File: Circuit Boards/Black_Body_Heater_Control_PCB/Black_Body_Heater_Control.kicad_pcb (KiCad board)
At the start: 2 copper layers, 57.5 x 42.8 mm, 57 parts, among them J201 5040500891, J202 Conn_01x04_Pin, J203 USB_C_Receptacle_USB2.0_16P, P301 436500200, P302 436500200, Q302 BD139, SW201 SW_MEC_5E, SW202 SW_MEC_5E, U201 AMS1117-3.3, U202 ESP32-S3-WROOM-1-N8R8, U203 USBLC6-2SC6, U301 DAC60501ZDGSR, U302 INA181A2IDBVR, U304 LMR51420XFDDCR, U305 LM358

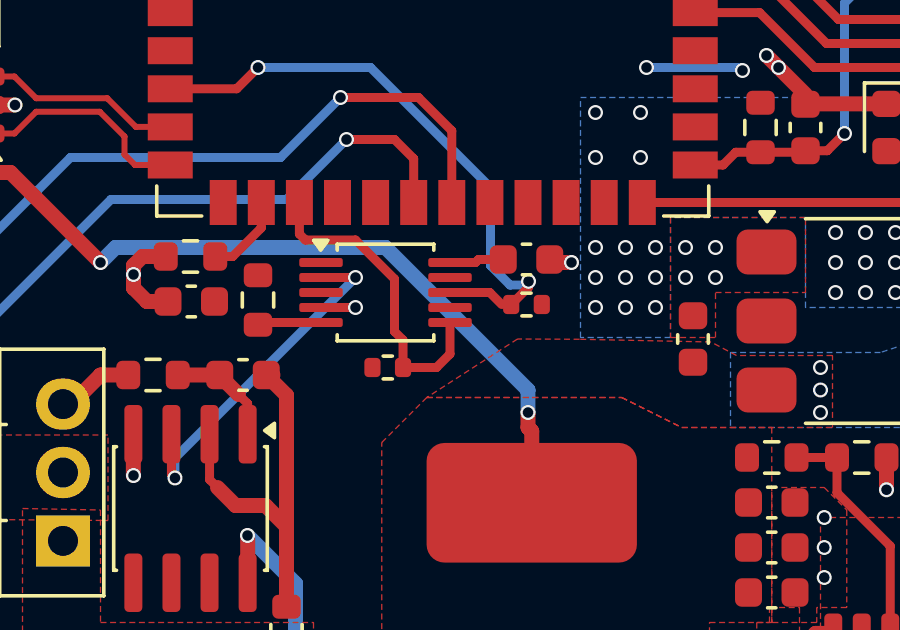
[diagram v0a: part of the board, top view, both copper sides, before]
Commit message: Minor pcb changes
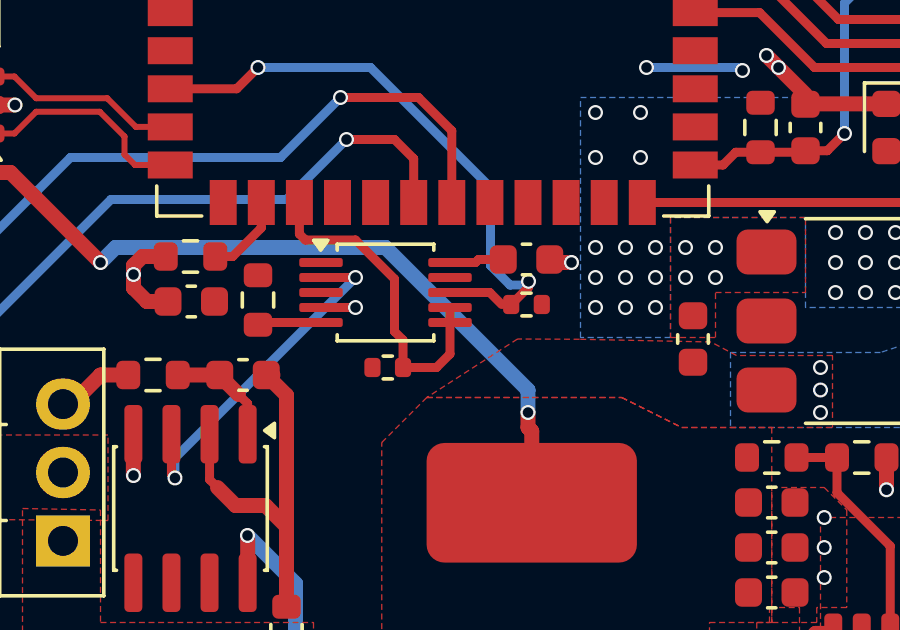
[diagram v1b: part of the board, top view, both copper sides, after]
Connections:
- U301 pad 7: unconnected-(U301-~{SYNC}/A0-Pad7) -> /ESP32/i2c.scl
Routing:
- net /ESP32/i2c.scl: track 10.7 -> 11.2 mm
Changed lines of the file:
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@@
 			(layers "F.Cu" "F.Mask" "F.Paste")
 			(roundrect_rratio 0.25)
-			(net "unconnected-(U301-~{SYNC}{slash}A0-Pad7)")
+			(net "/ESP32/i2c.scl")
 			(pinfunction "~{SYNC}/A0_7")
-			(pintype "input+no_connect")
+			(pintype "input")
 		)
 		(pad "8" smd roundrect
@@
 		(width 0.3)
 		(layer "F.Cu")
+		(net "/ESP32/i2c.scl")
+	)
+	(segment
+		(start 110.65 103.5)
+		(end 110.65 103)
+		(width 0.3)
+		(layer "F.Cu")
